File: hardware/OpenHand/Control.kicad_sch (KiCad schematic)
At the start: 48 parts, among them U10 DRV8833PWP, U11 DRV8833PWP, U12 DRV8833PWP, U9 DRV8833PWP

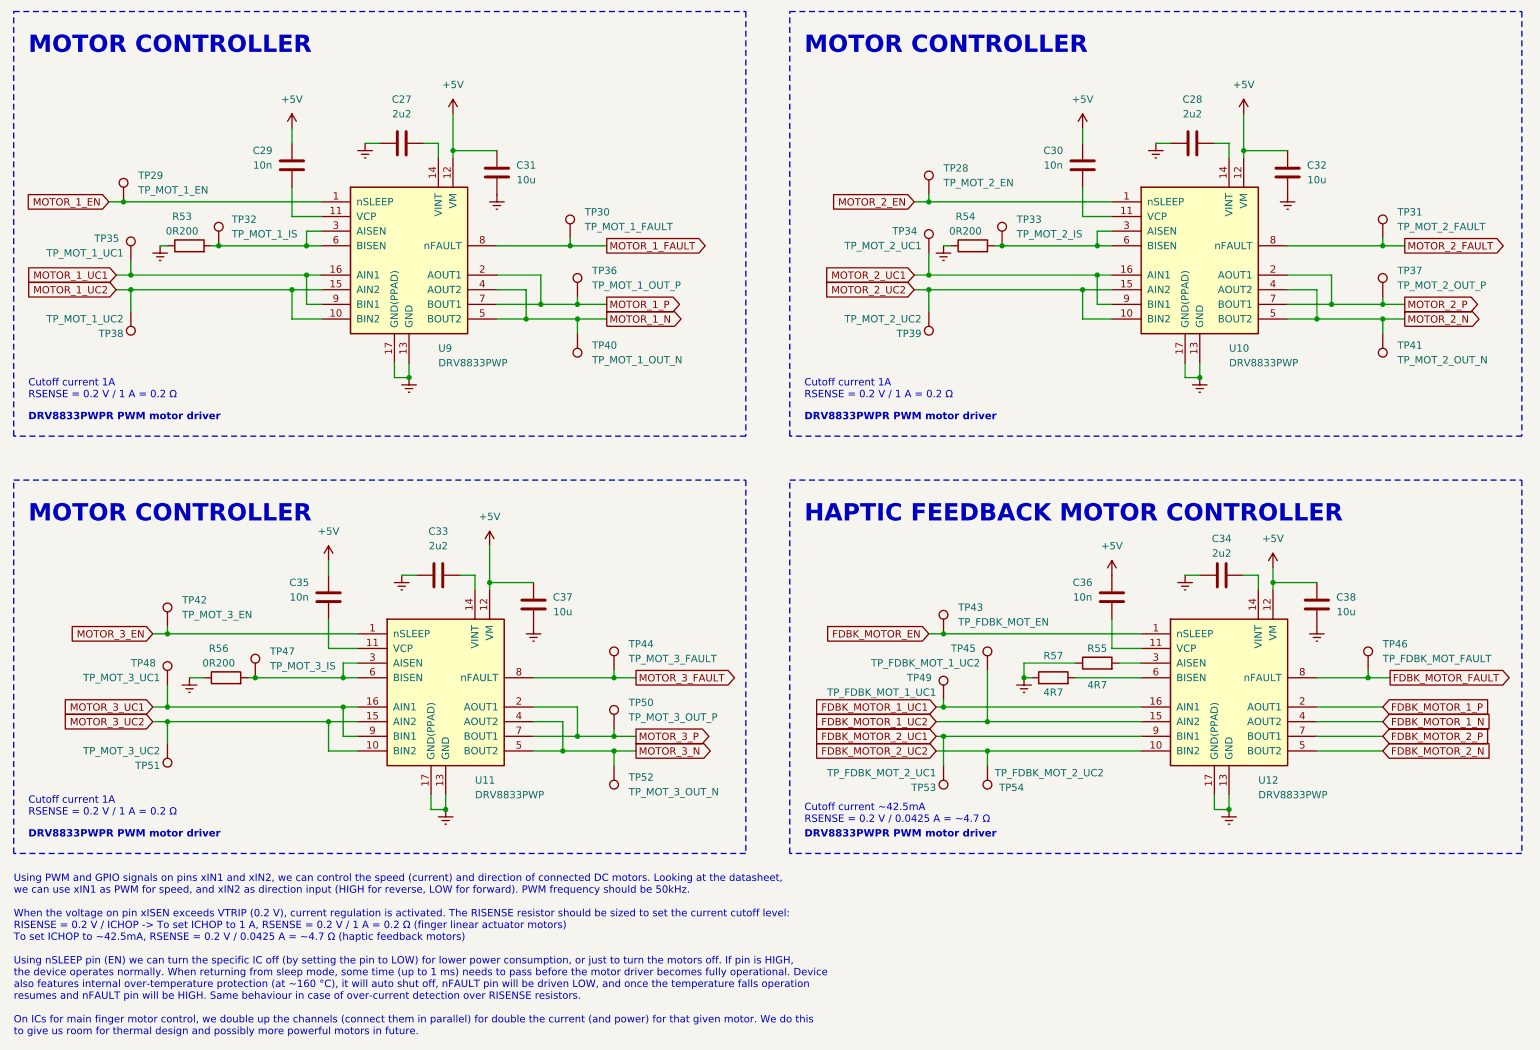
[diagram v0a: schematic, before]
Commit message: Update schm
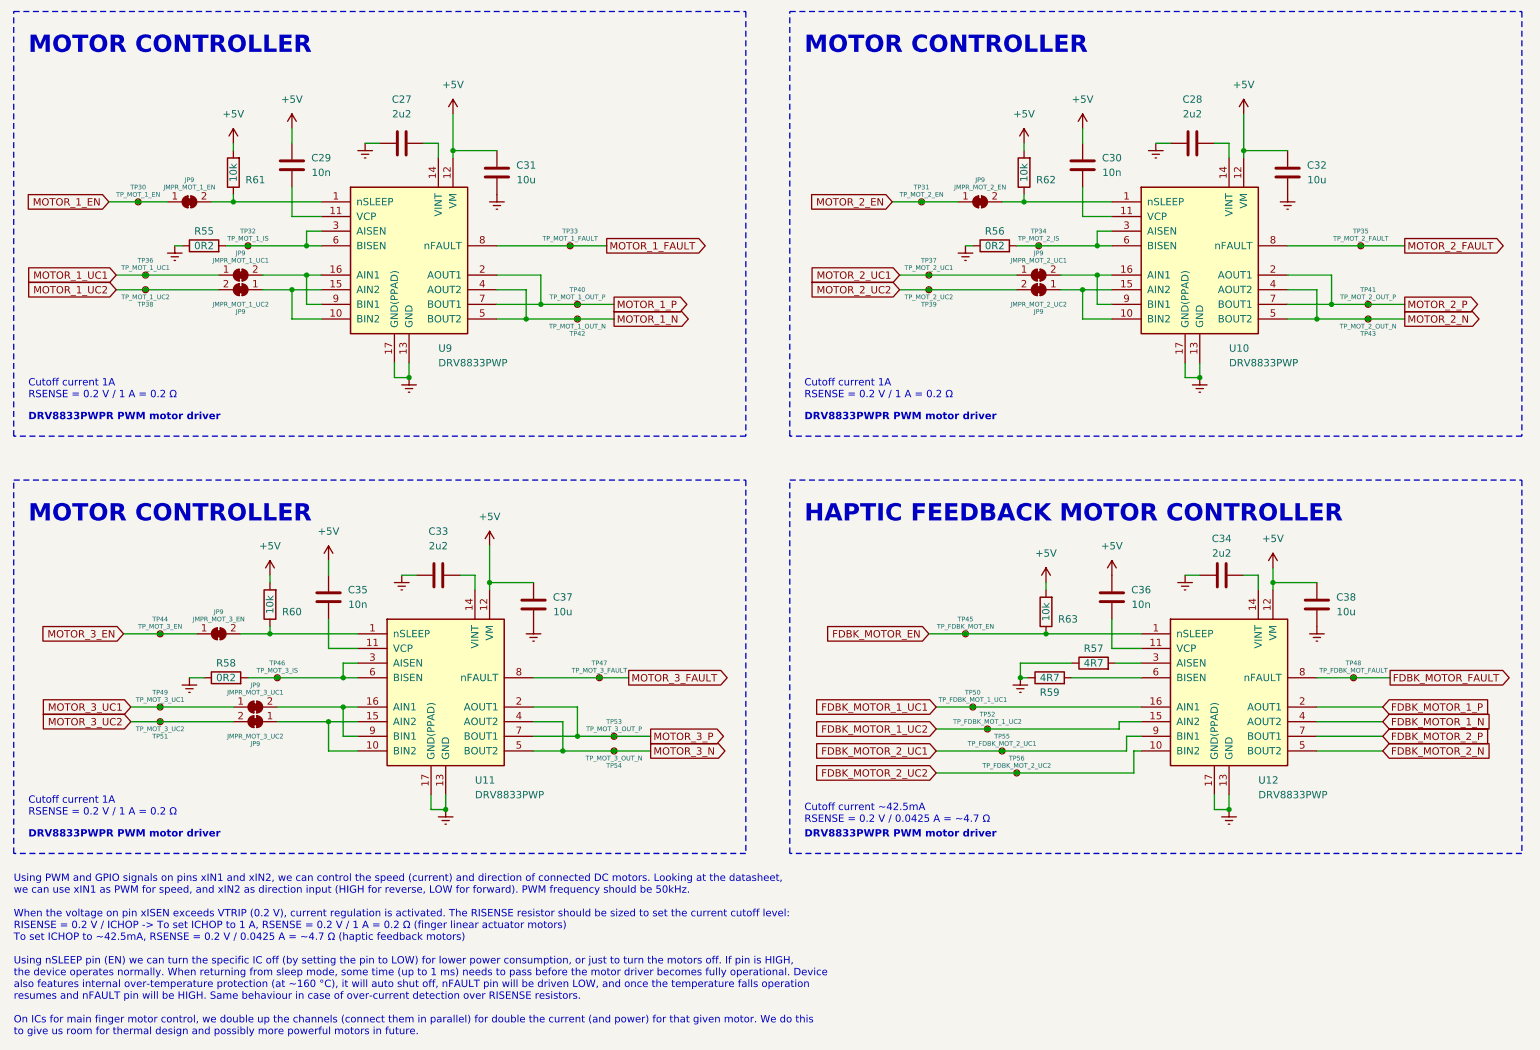
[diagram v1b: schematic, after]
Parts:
- removed TP28: TP_MOT_2_EN, TestPoint:TestPoint_Pad_D1.0mm, symbol Connector:TestPoint
- removed TP29: TP_MOT_1_EN, TestPoint:TestPoint_Pad_D1.0mm, symbol Connector:TestPoint
- removed TP30: TP_MOT_1_FAULT, TestPoint:TestPoint_Pad_D1.0mm, symbol Connector:TestPoint
- removed TP31: TP_MOT_2_FAULT, TestPoint:TestPoint_Pad_D1.0mm, symbol Connector:TestPoint
- removed TP32: TP_MOT_1_IS, TestPoint:TestPoint_Pad_D1.0mm, symbol Connector:TestPoint
- removed TP33: TP_MOT_2_IS, TestPoint:TestPoint_Pad_D1.0mm, symbol Connector:TestPoint
- removed TP34: TP_MOT_2_UC1, TestPoint:TestPoint_Pad_D1.0mm, symbol Connector:TestPoint
- removed TP35: TP_MOT_1_UC1, TestPoint:TestPoint_Pad_D1.0mm, symbol Connector:TestPoint
- removed TP36: TP_MOT_1_OUT_P, TestPoint:TestPoint_Pad_D1.0mm, symbol Connector:TestPoint
- removed TP37: TP_MOT_2_OUT_P, TestPoint:TestPoint_Pad_D1.0mm, symbol Connector:TestPoint
- removed TP38: TP_MOT_1_UC2, TestPoint:TestPoint_Pad_D1.0mm, symbol Connector:TestPoint
- removed TP39: TP_MOT_2_UC2, TestPoint:TestPoint_Pad_D1.0mm, symbol Connector:TestPoint
- removed TP40: TP_MOT_1_OUT_N, TestPoint:TestPoint_Pad_D1.0mm, symbol Connector:TestPoint
- removed TP41: TP_MOT_2_OUT_N, TestPoint:TestPoint_Pad_D1.0mm, symbol Connector:TestPoint
- removed TP42: TP_MOT_3_EN, TestPoint:TestPoint_Pad_D1.0mm, symbol Connector:TestPoint
- removed TP43: TP_FDBK_MOT_EN, TestPoint:TestPoint_Pad_D1.0mm, symbol Connector:TestPoint
- removed TP44: TP_MOT_3_FAULT, TestPoint:TestPoint_Pad_D1.0mm, symbol Connector:TestPoint
- removed TP45: TP_FDBK_MOT_1_UC2, TestPoint:TestPoint_Pad_D1.0mm, symbol Connector:TestPoint
- removed TP46: TP_FDBK_MOT_FAULT, TestPoint:TestPoint_Pad_D1.0mm, symbol Connector:TestPoint
- removed TP47: TP_MOT_3_IS, TestPoint:TestPoint_Pad_D1.0mm, symbol Connector:TestPoint
- removed TP48: TP_MOT_3_UC1, TestPoint:TestPoint_Pad_D1.0mm, symbol Connector:TestPoint
- removed TP49: TP_FDBK_MOT_1_UC1, TestPoint:TestPoint_Pad_D1.0mm, symbol Connector:TestPoint
- removed TP50: TP_MOT_3_OUT_P, TestPoint:TestPoint_Pad_D1.0mm, symbol Connector:TestPoint
- removed TP51: TP_MOT_3_UC2, TestPoint:TestPoint_Pad_D1.0mm, symbol Connector:TestPoint
- removed TP52: TP_MOT_3_OUT_N, TestPoint:TestPoint_Pad_D1.0mm, symbol Connector:TestPoint
- removed TP53: TP_FDBK_MOT_2_UC1, TestPoint:TestPoint_Pad_D1.0mm, symbol Connector:TestPoint
- removed TP54: TP_FDBK_MOT_2_UC2, TestPoint:TestPoint_Pad_D1.0mm, symbol Connector:TestPoint
- added JP9: JMPR_MOT_3_UC1, Jumper:SolderJumper-2_P1.3mm_Bridged_RoundedPad1.0x1.5mm, symbol Jumper:SolderJumper_2_Bridged
- added JP9: JMPR_MOT_1_EN, Jumper:SolderJumper-2_P1.3mm_Bridged_RoundedPad1.0x1.5mm, symbol Jumper:SolderJumper_2_Bridged
- added JP9: JMPR_MOT_1_UC1, Jumper:SolderJumper-2_P1.3mm_Bridged_RoundedPad1.0x1.5mm, symbol Jumper:SolderJumper_2_Bridged
- added JP9: JMPR_MOT_2_UC1, Jumper:SolderJumper-2_P1.3mm_Bridged_RoundedPad1.0x1.5mm, symbol Jumper:SolderJumper_2_Bridged
- added JP9: JMPR_MOT_2_EN, Jumper:SolderJumper-2_P1.3mm_Bridged_RoundedPad1.0x1.5mm, symbol Jumper:SolderJumper_2_Bridged
- added JP9: JMPR_MOT_1_UC2, Jumper:SolderJumper-2_P1.3mm_Bridged_RoundedPad1.0x1.5mm, symbol Jumper:SolderJumper_2_Bridged
- added JP9: JMPR_MOT_3_UC2, Jumper:SolderJumper-2_P1.3mm_Bridged_RoundedPad1.0x1.5mm, symbol Jumper:SolderJumper_2_Bridged
- added JP9: JMPR_MOT_3_EN, Jumper:SolderJumper-2_P1.3mm_Bridged_RoundedPad1.0x1.5mm, symbol Jumper:SolderJumper_2_Bridged
- added JP9: JMPR_MOT_2_UC2, Jumper:SolderJumper-2_P1.3mm_Bridged_RoundedPad1.0x1.5mm, symbol Jumper:SolderJumper_2_Bridged
- added R60, R61, R62, R63: 10k, Resistor_SMD:R_1206_3216Metric_Pad1.30x1.75mm_HandSolder, symbol Device:R
- added TP30: TP_MOT_1_EN, symbol Connector:TestPoint_Small
- added TP31: TP_MOT_2_EN, symbol Connector:TestPoint_Small
- added TP32: TP_MOT_1_IS, symbol Connector:TestPoint_Small
- added TP33: TP_MOT_1_FAULT, symbol Connector:TestPoint_Small
- added TP34: TP_MOT_2_IS, symbol Connector:TestPoint_Small
- added TP35: TP_MOT_2_FAULT, symbol Connector:TestPoint_Small
- added TP36: TP_MOT_1_UC1, symbol Connector:TestPoint_Small
- added TP37: TP_MOT_2_UC1, symbol Connector:TestPoint_Small
- added TP38: TP_MOT_1_UC2, symbol Connector:TestPoint_Small
- added TP39: TP_MOT_2_UC2, symbol Connector:TestPoint_Small
- added TP40: TP_MOT_1_OUT_P, symbol Connector:TestPoint_Small
- added TP41: TP_MOT_2_OUT_P, symbol Connector:TestPoint_Small
- added TP42: TP_MOT_1_OUT_N, symbol Connector:TestPoint_Small
- added TP43: TP_MOT_2_OUT_N, symbol Connector:TestPoint_Small
- added TP44: TP_MOT_3_EN, symbol Connector:TestPoint_Small
- added TP45: TP_FDBK_MOT_EN, symbol Connector:TestPoint_Small
- added TP46: TP_MOT_3_IS, symbol Connector:TestPoint_Small
- added TP47: TP_MOT_3_FAULT, symbol Connector:TestPoint_Small
- added TP48: TP_FDBK_MOT_FAULT, symbol Connector:TestPoint_Small
- added TP49: TP_MOT_3_UC1, symbol Connector:TestPoint_Small
- added TP50: TP_FDBK_MOT_1_UC1, symbol Connector:TestPoint_Small
- added TP51: TP_MOT_3_UC2, symbol Connector:TestPoint_Small
- added TP52: TP_FDBK_MOT_1_UC2, symbol Connector:TestPoint_Small
- added TP53: TP_MOT_3_OUT_P, symbol Connector:TestPoint_Small
- added TP54: TP_MOT_3_OUT_N, symbol Connector:TestPoint_Small
- added TP55: TP_FDBK_MOT_2_UC1, symbol Connector:TestPoint_Small
- added TP56: TP_FDBK_MOT_2_UC2, symbol Connector:TestPoint_Small
- R55: renamed from R53; value 0R200 -> 0R2
- R56: renamed from R54; value 0R200 -> 0R2
- R58: renamed from R56; value 0R200 -> 0R2
- renumbered R55 to R57, R57 to R59
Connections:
- net +5V: now also R60.2, R61.2, R62.2, R63.2
- net FDBK_MOTOR_1_UC1: now also TP50.1
- net FDBK_MOTOR_1_UC2: now also TP52.1
- net FDBK_MOTOR_2_UC1: now also TP55.1
- net FDBK_MOTOR_2_UC2: now also TP56.1
- net FDBK_MOTOR_EN: now also R63.1, TP45.1
- net FDBK_MOTOR_FAULT: now also TP48.1
- net MOTOR_1_EN: now also JP9.1 (A), TP30.1; no longer U9.1 (nSLEEP)
- net MOTOR_1_FAULT: now also TP33.1
- net MOTOR_1_N: now also TP42.1
- net MOTOR_1_P: now also TP40.1
- net MOTOR_1_UC1: now also JP9.1 (A), TP36.1; no longer U9.16 (AIN1), U9.9 (BIN1)
- net MOTOR_1_UC2: now also JP9.2 (B), TP38.1; no longer U9.10 (BIN2), U9.15 (AIN2)
- net MOTOR_2_EN: now also JP9.1 (A), TP31.1; no longer U10.1 (nSLEEP)
- net MOTOR_2_FAULT: now also TP35.1
- net MOTOR_2_N: now also TP43.1
- net MOTOR_2_P: now also TP41.1
- net MOTOR_2_UC1: now also JP9.1 (A), TP37.1; no longer U10.16 (AIN1), U10.9 (BIN1)
- net MOTOR_2_UC2: now also JP9.2 (B), TP39.1; no longer U10.10 (BIN2), U10.15 (AIN2)
- net MOTOR_3_EN: now also JP9.1 (A), TP44.1; no longer U11.1 (nSLEEP)
- net MOTOR_3_FAULT: now also TP47.1
- net MOTOR_3_N: now also TP54.1
- net MOTOR_3_P: now also TP53.1
- net MOTOR_3_UC1: now also JP9.1 (A), TP49.1; no longer U11.16 (AIN1), U11.9 (BIN1)
- net MOTOR_3_UC2: now also JP9.2 (B), TP51.1; no longer U11.10 (BIN2), U11.15 (AIN2)
- net at R58.2, U11.3 (AISEN), U11.6 (BISEN): now also TP46.1
- net at R56.2, U10.3 (AISEN), U10.6 (BISEN): now also TP34.1
- net at R55.2, U9.3 (AISEN), U9.6 (BISEN): now also TP32.1
- new net: JP9.2 (B), U11.16 (AIN1), U11.9 (BIN1)
- new net: JP9.2 (B), R60.1, U11.1 (nSLEEP)
- new net: JP9.1 (A), U11.10 (BIN2), U11.15 (AIN2)
- new net: JP9.2 (B), R62.1, U10.1 (nSLEEP)
- new net: JP9.1 (A), U10.10 (BIN2), U10.15 (AIN2)
- new net: JP9.2 (B), U10.16 (AIN1), U10.9 (BIN1)
- new net: JP9.2 (B), R61.1, U9.1 (nSLEEP)
- new net: JP9.2 (B), U9.16 (AIN1), U9.9 (BIN1)
- new net: JP9.1 (A), U9.10 (BIN2), U9.15 (AIN2)
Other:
- moved on the sheet: R55, R56, R57, R59
